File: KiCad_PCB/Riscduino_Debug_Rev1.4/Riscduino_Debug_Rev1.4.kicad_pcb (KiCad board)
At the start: 2 copper layers, 76.7 x 53.6 mm, 93 parts, among them J1 Conn_01x06_Pin, J10 Conn_01x08_Pin, J11 Conn_01x10_Pin, J12 Conn_01x03_Pin, J13 Conn_01x01, J2 ISP, J3 Conn_01x08_Pin, J4 Conn_01x01, J5 Conn_01x01, J6 Conn_02x04_Odd_Even, J7 Conn_01x08_Pin, J8 Conn_01x01, J9 USB_B_Micro, SW1 4Pin Round Button SPST Straig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, U1 APX811-29UG-7, U2 W25Q32JVSS, U3 23LC1024-I/P, U4 caravel-M.2-card, U5 CH340C, U6 LM1117MP-3.3, U7 LM1117S-ADJ, U8 W25Q32JVSS, X1 ASE-10.000MHZ-LC-T

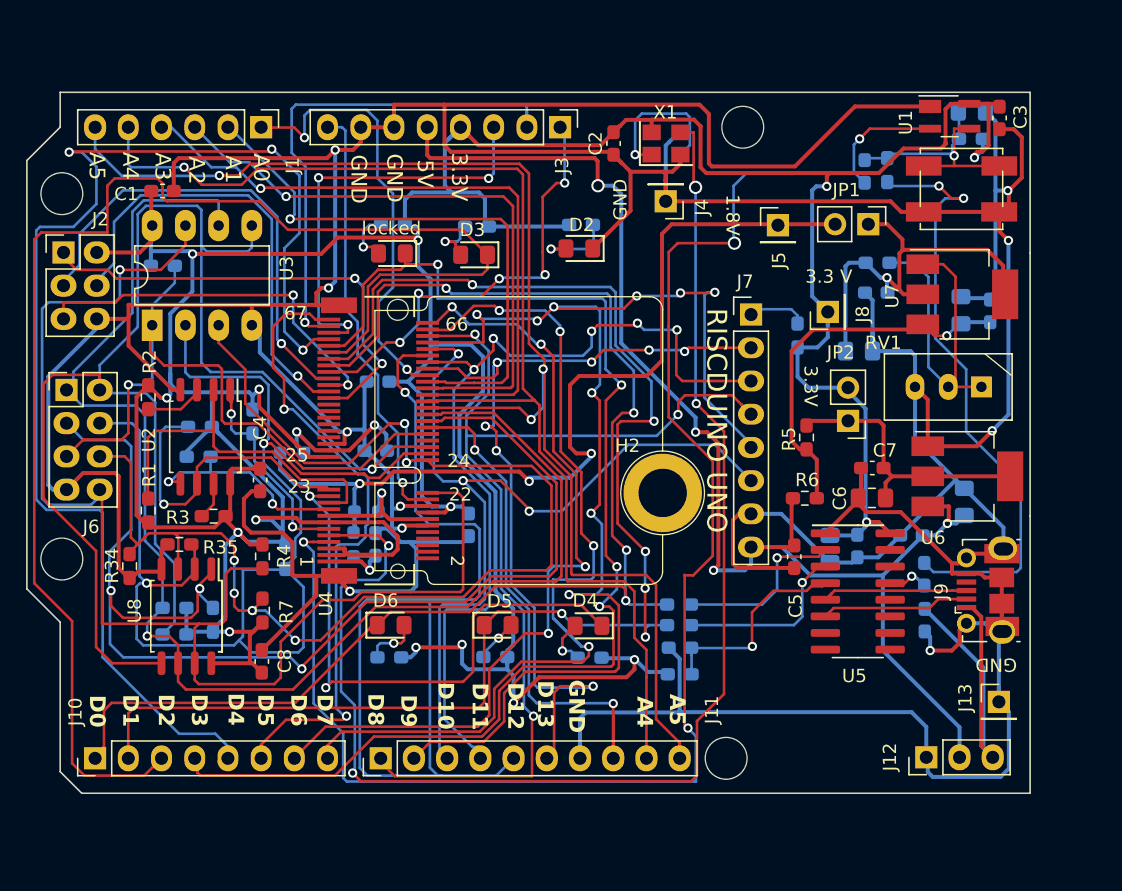
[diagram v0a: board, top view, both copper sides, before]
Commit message: update
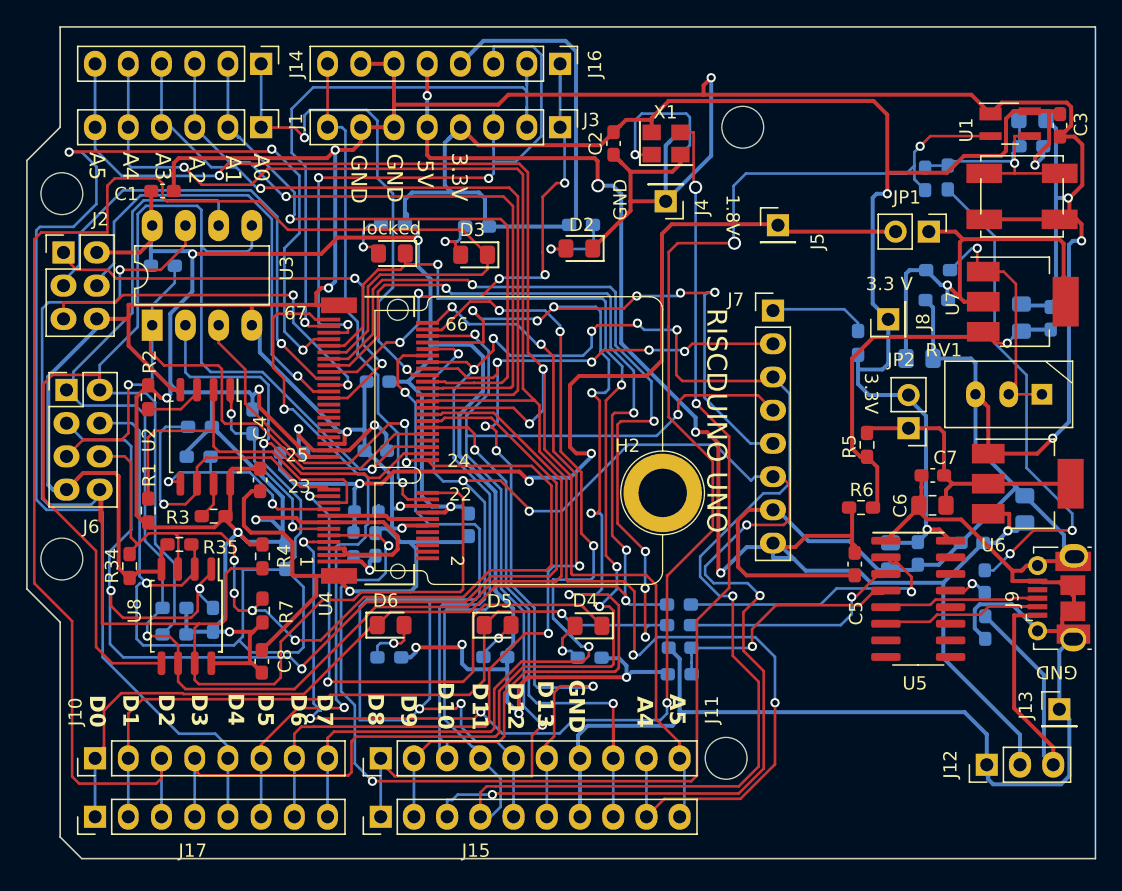
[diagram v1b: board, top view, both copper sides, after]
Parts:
- added J14: Conn_01x06_Male_Header, Riscduino.Library:PinHeader_1x06_P2.54mm_Vertical, F.Cu at (87.2, 47.3)
- added J15: Conn_01x10_Male_Header, Riscduino.Library:PinHeader_1x10_P2.54mm_Vertical, F.Cu at (96.3, 104.9)
- added J16: Conn_01x08_Male_Header, Riscduino.Library:PinHeader_1x08_P2.54mm_Vertical, F.Cu at (110.1, 47.3)
- added J17: Conn_01x08_Male_Header, Riscduino.Library:PinHeader_1x08_P2.54mm_Vertical, F.Cu at (74.5, 104.9)
- J1: value Conn_01x06_Pin -> Conn_01x06_Female_Header
- J10, J3: value Conn_01x08_Pin -> Conn_01x08_Female_Header
- J11: value Conn_01x10_Pin -> Conn_01x10_Female_Header
- moved J9 5.47 mm to (148.0, 88.2)
- moved R17 4.66 mm to (132.8, 68.7)
- moved R12 4.66 mm to (139.0, 63.1)
- moved U1 4.66 mm to (144.5, 51.9)
- moved C11 4.66 mm to (145.6, 81.4)
- moved C12 4.66 mm to (147.6, 66.8)
- moved C13 4.66 mm to (135.3, 85.0)
- moved C23 4.66 mm to (142.6, 90.4)
- moved C3 4.66 mm to (148.3, 52.0)
- moved J12 4.66 mm to (142.7, 100.9)
- moved J8 4.66 mm to (135.2, 66.9)
- moved R10 4.66 mm to (138.0, 56.1)
- moved C5 4.66 mm to (132.6, 85.6)
- moved C15 4.66 mm to (142.5, 86.9)
- moved C18 4.66 mm to (137.4, 84.8)
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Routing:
- net ardunio_d11: track 68.5 -> 134.9 mm, vias 5 -> 6
- net ardunio_d10: track 66.2 -> 126.5 mm, vias 3 -> 6
- net ardunio_a4: track 93.6 -> 126.5 mm, vias 1 -> 3
- net +3.3V: track 367.0 -> 397.8 mm
- net mprj_io_11: track 34.3 -> 51.1 mm
- net +5V: track 101.3 -> 115.1 mm, vias 4 -> 5
- net GND: track 483.1 -> 494.8 mm
- net ardunio_d9: track 97.7 -> 107.6 mm
- net Net-(U5-TXD): track 13.4 -> 22.3 mm
- net Net-(C15-Pad2): track 45.9 -> 38.0 mm
- net ardunio_a5: track 102.4 -> 110.1 mm
- net Net-(U7-ADJ): track 25.8 -> 18.2 mm, vias 0 -> 1
- net ardunio_d13: track 66.2 -> 73.5 mm
- net mprj_io_5_ser_rx: track 32.9 -> 39.9 mm
- net ardunio_d3: track 96.8 -> 103.3 mm
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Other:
- board size 76.7 x 53.6 mm -> 81.7 x 63.6 mm
